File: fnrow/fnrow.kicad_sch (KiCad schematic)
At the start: 54 parts, among them J1 USB_C_Receptacle_USB2.0, J2 Conn_01x04, SW1 SW_Push, SW10 SW_Push, SW11 SW_Push, SW12 SW_Push, SW13 SW_Push, SW14 SW_Push, SW2 SW_Push, SW3 SW_Push, SW4 SW_Push, SW5 SW_Push, SW6 SW_Push, SW7 SW_Push, SW8 SW_Push, SW9 SW_Push, U1 LD1117S33TR_SOT223, U2 USB6B1, U3 STM32F042K6Tx

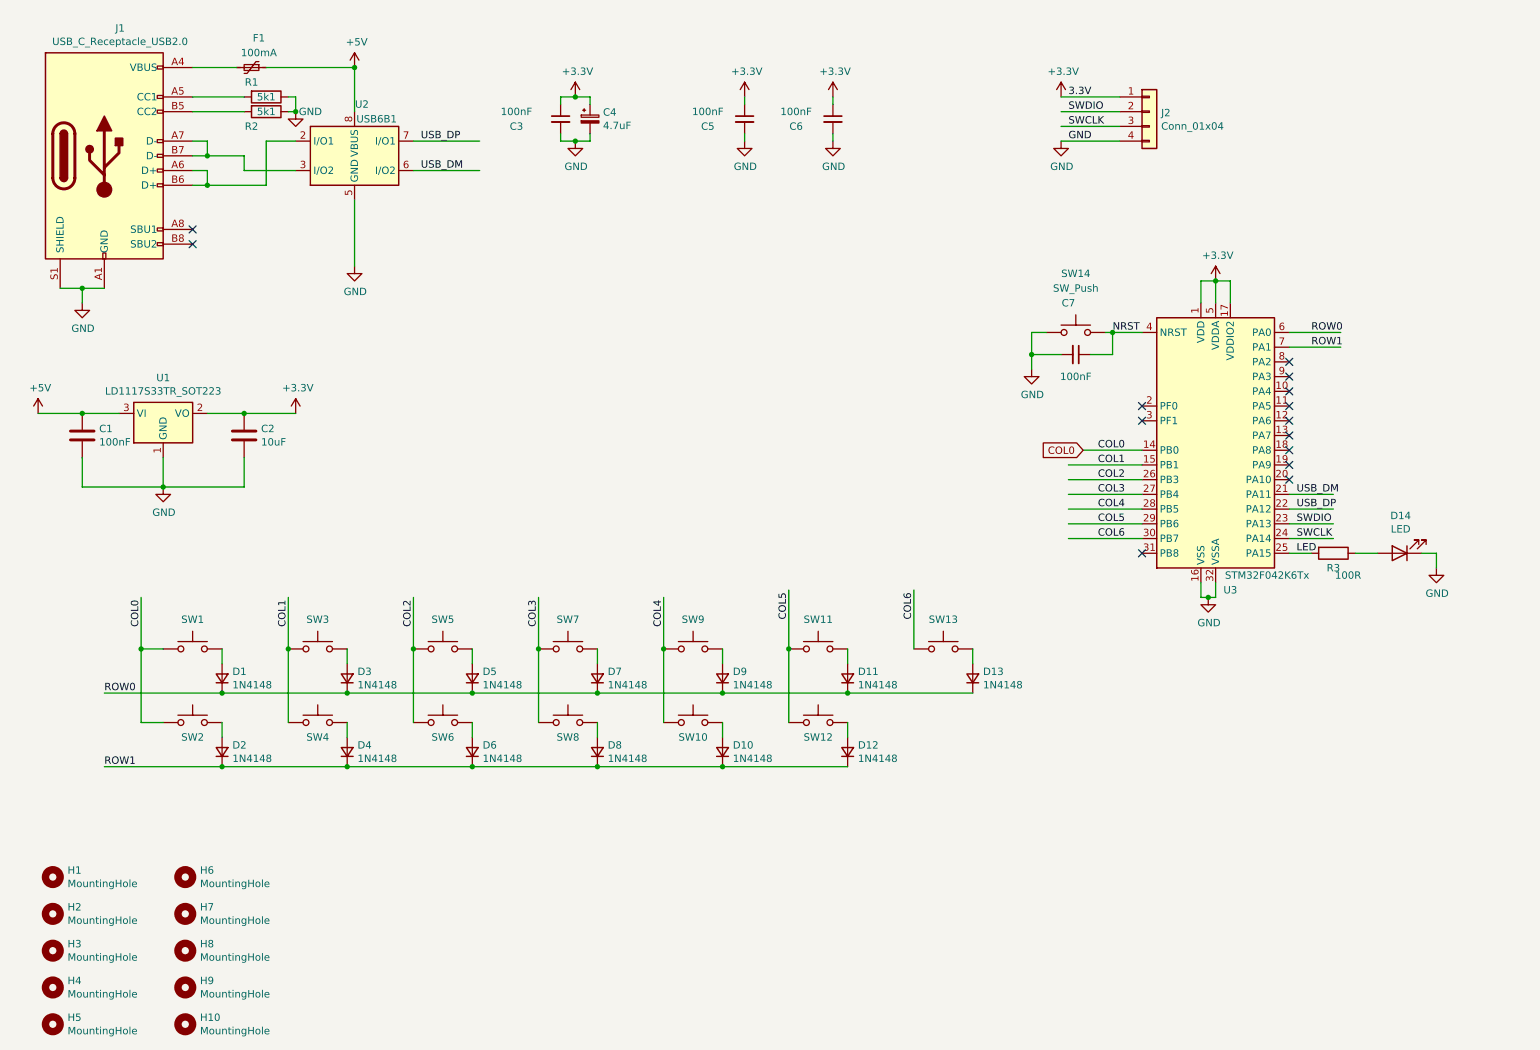
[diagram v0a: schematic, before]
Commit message: WIP
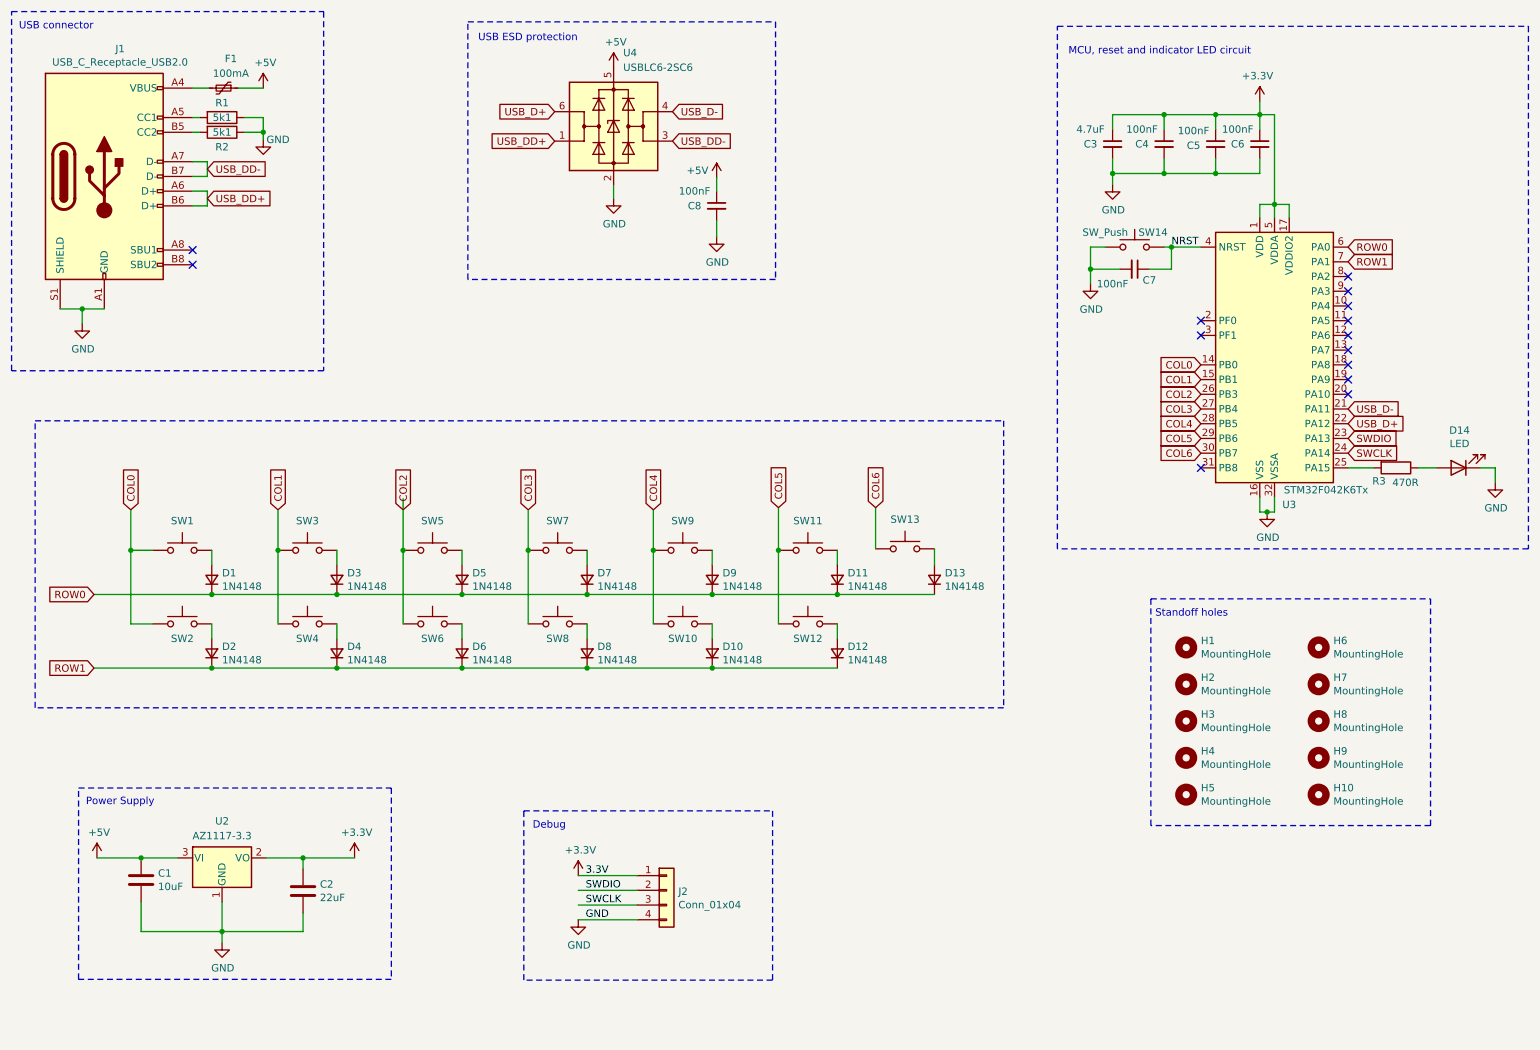
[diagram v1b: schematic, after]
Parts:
- removed C4: 4.7uF, Capacitor_Tantalum_SMD:CP_EIA-3216-12_Kemet-S_Pad1.58x1.35mm_HandSolder, symbol fnrow-rescue:CP_Small-Device
- removed U1: LD1117S33TR_SOT223, Package_TO_SOT_SMD:SOT-223-3_TabPin2, symbol Regulator_Linear:LD1117S33TR_SOT223
- removed U2: USB6B1, Package_SO:SOIC-8_3.9x4.9mm_P1.27mm, symbol Power_Protection:USB6B1
- added C4, C8: 100nF, Capacitor_SMD:C_0402_1005Metric, symbol Device:C_Small
- added U2: AZ1117-3.3, Package_TO_SOT_SMD:SOT-223, symbol Regulator_Linear:AZ1117-3.3
- added U4: USBLC6-2SC6, Package_TO_SOT_SMD:SOT-23-6, symbol Power_Protection:USBLC6-2P6
- C1: value 100nF -> 10uF; footprint Capacitor_SMD:C_0603_1608Metric_Pad1.08x0.95mm_HandSolder -> Capacitor_SMD:C_0805_2012Metric
- C2: value 10uF -> 22uF; footprint Capacitor_Tantalum_SMD:CP_EIA-3216-12_Kemet-S_Pad1.58x1.35mm_HandSolder -> Capacitor_SMD:C_0805_2012Metric
- C3: value 100nF -> 4.7uF; footprint Capacitor_SMD:C_0603_1608Metric_Pad1.08x0.95mm_HandSolder -> Capacitor_SMD:C_0603_1608Metric
- C5, C6, C7: footprint Capacitor_SMD:C_0603_1608Metric_Pad1.08x0.95mm_HandSolder -> Capacitor_SMD:C_0402_1005Metric
- D14: footprint LED_SMD:LED_0805_2012Metric_Pad1.15x1.40mm_HandSolder -> LED_SMD:LED_0805_2012Metric
- F1: footprint Fuse:Fuse_0805_2012Metric_Pad1.15x1.40mm_HandSolder -> Fuse:Fuse_0805_2012Metric; LCSC (none) -> C2687880
- J1: footprint Connector_USB:USB_C_Receptacle_GCT_USB4085 -> Connector_USB:USB_C_Receptacle_HRO_TYPE-C-31-M-12; LCSC (none) -> C2689845
- R1, R2: footprint Resistor_SMD:R_0603_1608Metric_Pad0.98x0.95mm_HandSolder -> Capacitor_SMD:C_0402_1005Metric
- R3: value 100R -> 470R; footprint Resistor_SMD:R_0603_1608Metric_Pad0.98x0.95mm_HandSolder -> Capacitor_SMD:C_0402_1005Metric
- SW14: footprint eec:Wuerth_Elektronik-434121043816-Manufacturer_Recommended -> Button_Switch_SMD:SW_Push_1P1T_XKB_TS-1187A; LCSC (none) -> C318884
- U3: LCSC (none) -> C69216
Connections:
- net +3V3: now also C4.1, U2.2 (VO)
- net +5V: now also C8.1, U2.3 (VI), U4.5 (VBUS)
- net GND: now also C4.2, C8.2, U2.1 (GND), U4.2 (GND)
- net USB_DD+: now reaches J1.A6 (D+), J1.B6 (D+)
- net USB_DD+: now also U4.1 (I/O1)
- net USB_DD-: now reaches J1.A7 (D-), J1.B7 (D-)
- net USB_DD-: now also U4.3 (I/O2)
- net LED: no longer names the net of R3.2, U3.25 (PA15)
- net USB_DM renamed USB_D-
- net USB_D-: now also U4.4 (I/O2)
- net USB_DP renamed USB_D+
- net USB_D+: now also U4.6 (I/O1)
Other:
- note added: "Debug"
- note added: "MCU, reset and indicator LED circuit"
- note added: "Power Supply"
- note added: "Standoff holes"
- note added: "USB ESD protection"
- note added: "USB connector"
- moved on the sheet: C1, C2, C3, C5, C6, C7, D1, D10, D11, D12, D13, D14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
